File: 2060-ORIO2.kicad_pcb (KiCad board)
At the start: 4 copper layers, 99 x 99 mm, 159 parts, among them J1 TBL001-500-02GY-2GY, J101 RaspberryPI-B+header, J133 Conn_02x05_Odd_Even, J134 Conn_01x04, J301 Conn_01x08, J302 Conn_01x08, J303 Conn_01x08, J304 Conn_01x08, J305 Conn_01x08, J306 Conn_01x08, J307 Conn_01x08, J308 Conn_01x08, J321 Conn_01x08, J322 Conn_01x08, J323 Conn_01x08, J331 Conn_01x08, J332 Conn_01x08, J333 Conn_01x08, J341 Conn_01x10, J342 Conn_01x10, J343 Conn_01x10, J35 Conn_01x02, J351 Conn_01x10, J352 Conn_01x10, J353 Conn_01x10, J354 Conn_01x10, Q101 DMG2305UX-13, Q102 ULN2803ADWR, Q103 DMMT5401, SW101 SW_DIP_x08, U1 TPS563231, U10 SN74LVC4245AN, U102 AZ1117CH-3.3TRG1, U103 AZ1117CH-1.2, U104 ICE40HX4K-TQ144, U105 MCP3008, U11 AZ1117CH-3.3TRG1, U12 AP3012, U2 TPS563231, U3 SN74LVC4245AN, U4 SN74LVC4245AN, U5 SN74LVC4245AN, U6 SN74LVC4245AN, U7 SN74LVC4245AN, U8 TPS563231, U9 SN74LVC4245AN, Y101 XLH536025_000000I

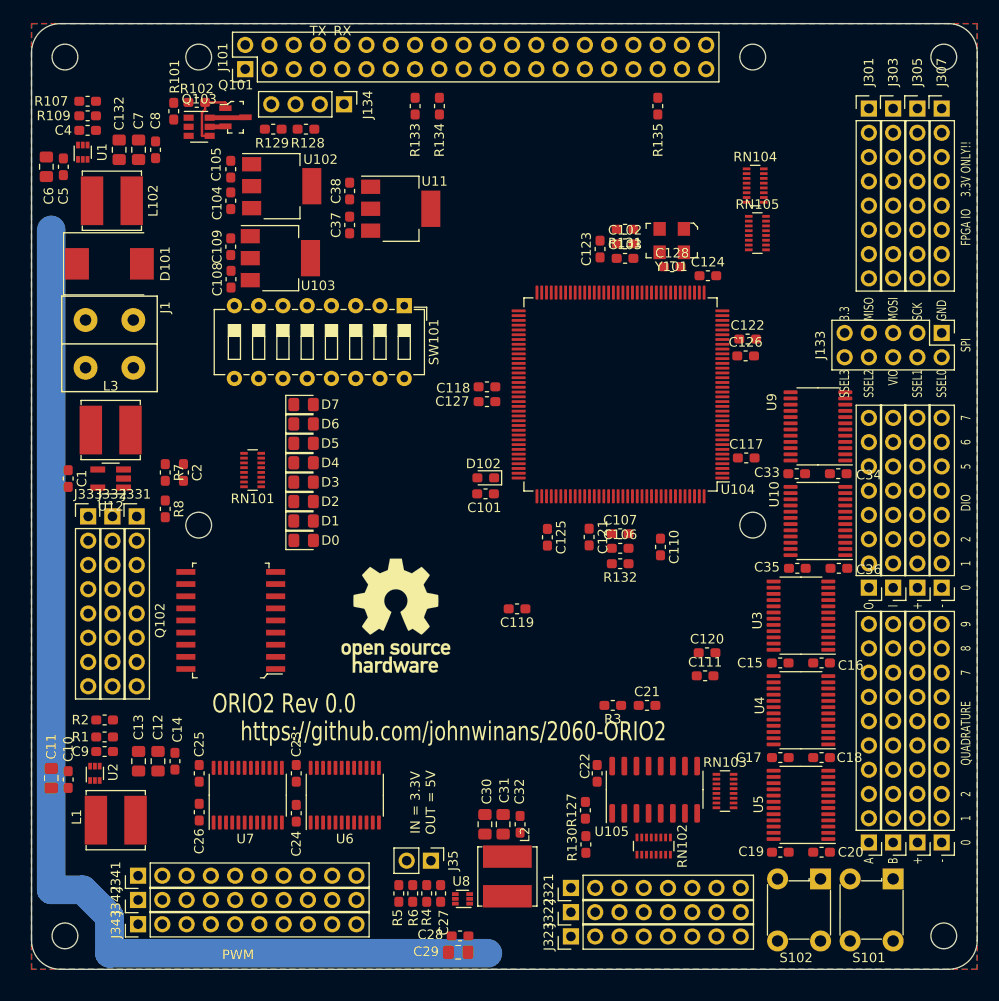
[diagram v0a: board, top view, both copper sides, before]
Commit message: checkpoint
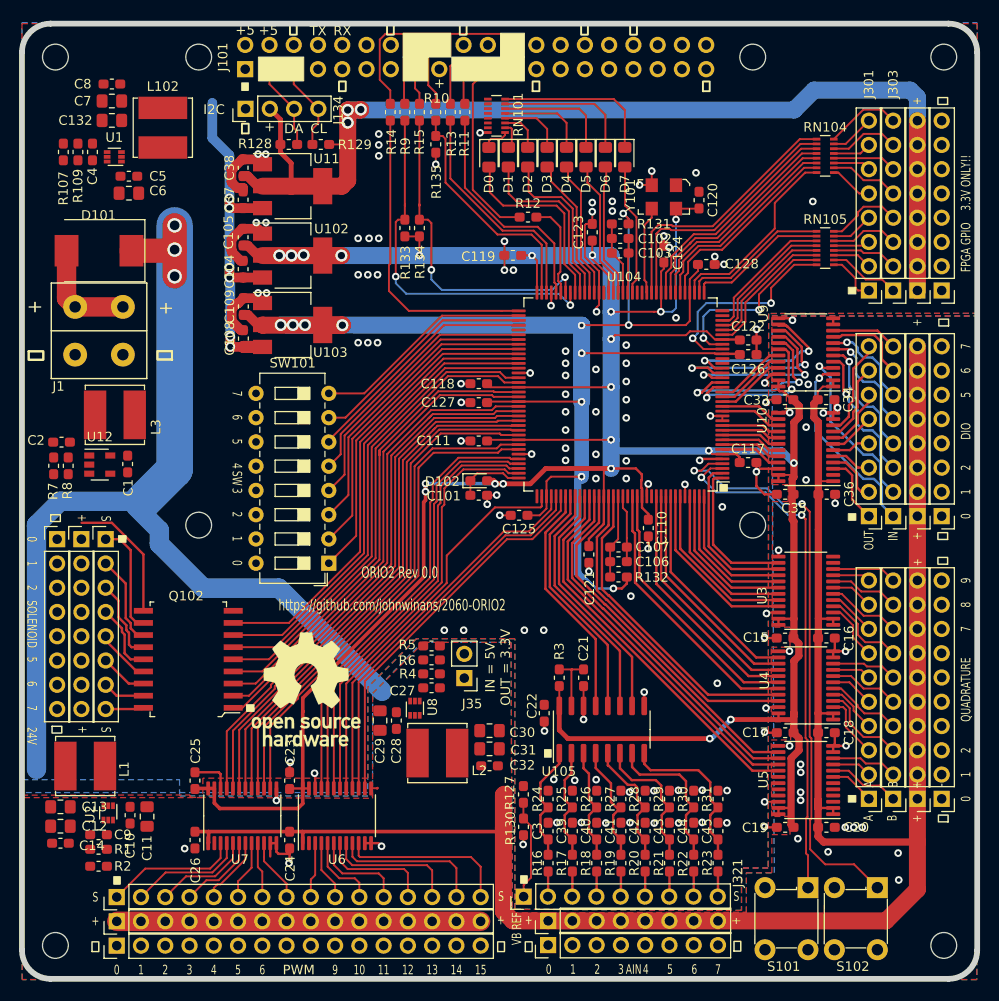
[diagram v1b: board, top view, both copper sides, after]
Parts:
- removed J133: Conn_02x05_Odd_Even, Connector_PinHeader_2.54mm:PinHeader_2x05_P2.54mm_Vertical
- removed Q101: DMG2305UX-13, digikey-footprints:SOT-23-3
- removed Q103: DMMT5401, Package_TO_SOT_SMD:SOT-23-6
- removed R101, R102: 22, Resistor_SMD:R_0603_1608Metric_Pad1.05x0.95mm_HandSolder
- removed RN102, RN103: R_Pack08, Resistor_SMD:R_Array_Convex_8x0602
- added C3: X, Capacitor_SMD:C_0603_1608Metric_Pad1.05x0.95mm_HandSolder, F.Cu at (127.1, 126.5)
- added C39: X, Capacitor_SMD:C_0603_1608Metric_Pad1.05x0.95mm_HandSolder, F.Cu at (129.6, 126.5)
- added C40: X, Capacitor_SMD:C_0603_1608Metric_Pad1.05x0.95mm_HandSolder, F.Cu at (132.2, 126.5)
- added C41: X, Capacitor_SMD:C_0603_1608Metric_Pad1.05x0.95mm_HandSolder, F.Cu at (134.7, 126.5)
- added C42: X, Capacitor_SMD:C_0603_1608Metric_Pad1.05x0.95mm_HandSolder, F.Cu at (137.2, 126.5)
- added C43: X, Capacitor_SMD:C_0603_1608Metric_Pad1.05x0.95mm_HandSolder, F.Cu at (139.8, 126.5)
- added C44: X, Capacitor_SMD:C_0603_1608Metric_Pad1.05x0.95mm_HandSolder, F.Cu at (142.3, 126.5)
- added C45: X, Capacitor_SMD:C_0603_1608Metric_Pad1.05x0.95mm_HandSolder, F.Cu at (144.9, 126.5)
- added R10: X, Resistor_SMD:R_0603_1608Metric_Pad1.05x0.95mm_HandSolder, F.Cu at (115.3, 51.3)
- added R11: X, Resistor_SMD:R_0603_1608Metric_Pad1.05x0.95mm_HandSolder, F.Cu at (118.4, 51.3)
- added R12: X, Resistor_SMD:R_0603_1608Metric_Pad1.05x0.95mm_HandSolder, F.Cu at (125.0, 62.3)
- added R13: X, Resistor_SMD:R_0603_1608Metric_Pad1.05x0.95mm_HandSolder, F.Cu at (116.8, 51.3)
- added R14: X, Resistor_SMD:R_0603_1608Metric_Pad1.05x0.95mm_HandSolder, F.Cu at (110.6, 51.3)
- added R15: X, Resistor_SMD:R_0603_1608Metric_Pad1.05x0.95mm_HandSolder, F.Cu at (113.6, 51.3)
- added R16: X, Resistor_SMD:R_0603_1608Metric_Pad1.05x0.95mm_HandSolder, F.Cu at (127.1, 129.9)
- added R17: X, Resistor_SMD:R_0603_1608Metric_Pad1.05x0.95mm_HandSolder, F.Cu at (129.6, 129.9)
- added R18: X, Resistor_SMD:R_0603_1608Metric_Pad1.05x0.95mm_HandSolder, F.Cu at (132.2, 129.9)
- added R19: X, Resistor_SMD:R_0603_1608Metric_Pad1.05x0.95mm_HandSolder, F.Cu at (134.7, 129.9)
- added R20: X, Resistor_SMD:R_0603_1608Metric_Pad1.05x0.95mm_HandSolder, F.Cu at (137.2, 129.9)
- added R21: X, Resistor_SMD:R_0603_1608Metric_Pad1.05x0.95mm_HandSolder, F.Cu at (139.8, 129.9)
- added R22: X, Resistor_SMD:R_0603_1608Metric_Pad1.05x0.95mm_HandSolder, F.Cu at (142.3, 129.9)
- added R23: X, Resistor_SMD:R_0603_1608Metric_Pad1.05x0.95mm_HandSolder, F.Cu at (144.9, 129.9)
- added R24: X, Resistor_SMD:R_0603_1608Metric_Pad1.05x0.95mm_HandSolder, F.Cu at (127.1, 123.2)
- added R25: X, Resistor_SMD:R_0603_1608Metric_Pad1.05x0.95mm_HandSolder, F.Cu at (129.6, 123.2)
- added R26: X, Resistor_SMD:R_0603_1608Metric_Pad1.05x0.95mm_HandSolder, F.Cu at (132.2, 123.2)
- added R27: X, Resistor_SMD:R_0603_1608Metric_Pad1.05x0.95mm_HandSolder, F.Cu at (134.7, 123.2)
- added R28: X, Resistor_SMD:R_0603_1608Metric_Pad1.05x0.95mm_HandSolder, F.Cu at (137.2, 123.2)
- added R29: X, Resistor_SMD:R_0603_1608Metric_Pad1.05x0.95mm_HandSolder, F.Cu at (139.8, 123.2)
- added R30: X, Resistor_SMD:R_0603_1608Metric_Pad1.05x0.95mm_HandSolder, F.Cu at (142.3, 123.2)
- added R31: X, Resistor_SMD:R_0603_1608Metric_Pad1.05x0.95mm_HandSolder, F.Cu at (144.9, 123.2)
- added R9: X, Resistor_SMD:R_0603_1608Metric_Pad1.05x0.95mm_HandSolder, F.Cu at (112.1, 51.3)
- J321: value Conn_01x08 -> Conn_01x09; footprint Connector_PinHeader_2.54mm:PinHeader_1x08_P2.54mm_Vertical -> Connector_PinHeader_2.54mm:PinHeader_1x09_P2.54mm_Vertical
- J341, J342, J343: value Conn_01x10 -> Conn_01x16; footprint Connector_PinHeader_2.54mm:PinHeader_1x10_P2.54mm_Vertical -> Connector_PinHeader_2.54mm:PinHeader_1x16_P2.54mm_Vertical
- U12: footprint Package_TO_SOT_SMD:SOT-23-5_HandSoldering -> Package_TO_SOT_SMD:SOT-23-5
- moved C120 47.4 mm to (142.9, 60.5), turned to 90 degrees
- moved RN101 45.0 mm to (121.7, 51.7)
- moved D0 44.6 mm to (120.9, 56.0), turned to 270 degrees
- moved D1 43.7 mm to (122.9, 56.0), turned to 270 degrees
- moved D2 43.0 mm to (124.9, 56.0), turned to 270 degrees
- moved D3 42.5 mm to (127.0, 56.0), turned to 270 degrees
- moved D7 42.4 mm to (135.1, 56.0), turned to 270 degrees
- moved D4 42.2 mm to (129.0, 56.0), turned to 270 degrees
- moved D6 42.2 mm to (133.1, 56.0), turned to 270 degrees
- moved D5 42.1 mm to (131.0, 56.0), turned to 270 degrees
- moved C119 37.0 mm to (123.4, 66.3)
- moved C111 34.1 mm to (119.8, 85.7), turned to 180 degrees
- moved SW101 28.1 mm to (104.1, 98.5), turned to 180 degrees
- moved R5 26.1 mm to (114.9, 107.2), turned to 0 degrees
- moved C29 25.6 mm to (109.5, 115.0), turned to 270 degrees
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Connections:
- net /IOT_197 renamed Net-(U104-Pad128)
- net Net-(J301-Pad6) renamed /FIO10
- net Net-(J303-Pad3) renamed /FIO5
- C22 pad 1: VCC_IO -> +3V3
- J101 pad 16: /CDONE -> /GPIO23
- J101 pad 18: /~CRESET~ -> /GPIO24
- J101 pad 19: /FPGA_MOSI -> /SPI_MOSI
- J101 pad 21: /FPGA_MISO -> /SPI_MISO
- J101 pad 23: /FPGA_SCLK -> /SPI_SCLK
- J101 pad 36: /FPGA_SSEL -> /GPIO16
- J301 pad 1: Net-(J301-Pad1) -> /FIO0
- J301 pad 2: Net-(J301-Pad2) -> /FIO2
- J301 pad 3: Net-(J301-Pad3) -> /FIO4
- J301 pad 4: Net-(J301-Pad4) -> /FIO6
- J301 pad 5: Net-(J301-Pad5) -> /FIO8
- J301 pad 7: Net-(J301-Pad7) -> /FIO12
- J301 pad 8: Net-(J301-Pad8) -> /FIO14
- J303 pad 1: Net-(J303-Pad1) -> /FIO1
- J303 pad 2: Net-(J303-Pad2) -> /FIO3
- J303 pad 4: Net-(J303-Pad4) -> /FIO7
- J303 pad 5: Net-(J303-Pad5) -> /FIO9
- J303 pad 6: Net-(J303-Pad6) -> /FIO11
- J303 pad 7: Net-(J303-Pad7) -> /FIO13
- J303 pad 8: Net-(J303-Pad8) -> /FIO15
- J321 pad 1: Net-(J321-Pad1) -> /VBATT_DIV
- J35 pad 1: VCC_IO -> Net-(J35-Pad1)
- J35 pad 2: Net-(J35-Pad2) -> GND
- J351 pad 4: /Qa3 -> /QA3
- R127 pad 1: /ADC0_11 -> /VBATT_DIV
- R130 pad 2: /ADC0_11 -> /VBATT_DIV
- R135 pad 2: /FPGA_SSEL -> /FPGA_SS
- R3 pad 2: VCC_IO -> +3V3
- R6 pad 1: Net-(J35-Pad2) -> Net-(J35-Pad1)
- RN104 pad 1: Net-(RN104-Pad1) -> /IOB_80
- RN104 pad 10: Net-(J301-Pad7) -> /FIO9
- RN104 pad 12: Net-(J301-Pad5) -> /FIO11
- RN104 pad 13: Net-(J301-Pad4) -> /FIO12
- RN104 pad 14: Net-(J301-Pad3) -> /FIO13
- RN104 pad 15: Net-(J301-Pad2) -> /FIO14
- RN104 pad 16: Net-(J301-Pad1) -> /FIO15
- RN104 pad 2: Net-(RN104-Pad2) -> /IOB_79
- RN104 pad 3: Net-(RN104-Pad3) -> /IOB_73
- RN104 pad 4: Net-(RN104-Pad4) -> /IOB_72
- RN104 pad 5: Net-(RN104-Pad5) -> /IOB_71
- RN104 pad 6: Net-(RN104-Pad6) -> /IOB_64
- RN104 pad 7: Net-(RN104-Pad7) -> /IOB_63
- RN104 pad 8: Net-(RN104-Pad8) -> /IOB_61
- RN104 pad 9: Net-(J301-Pad8) -> /FIO8
- RN105 pad 1: Net-(RN105-Pad1) -> /IOB_57
- RN105 pad 10: Net-(J303-Pad7) -> /FIO1
- RN105 pad 11: Net-(J303-Pad6) -> /FIO2
- RN105 pad 12: Net-(J303-Pad5) -> /FIO3
- RN105 pad 13: Net-(J303-Pad4) -> /FIO4
- RN105 pad 15: Net-(J303-Pad2) -> /FIO6
- RN105 pad 16: Net-(J303-Pad1) -> /FIO7
- RN105 pad 2: Net-(RN105-Pad2) -> /IOB_56
- RN105 pad 3: Net-(RN105-Pad3) -> /IOL_25B
- RN105 pad 4: Net-(RN105-Pad4) -> /IOL_25A
- RN105 pad 5: Net-(RN105-Pad5) -> /IOL_24B
- RN105 pad 6: Net-(RN105-Pad6) -> /IOL_24A
- RN105 pad 7: Net-(RN105-Pad7) -> /IOL_23B
- RN105 pad 8: Net-(RN105-Pad8) -> /IOL_23A
- RN105 pad 9: Net-(J303-Pad8) -> /FIO0
- S101 pad 1: /IOT_220 -> /PB0
- S101 pad 4: GND -> Net-(S101-Pad4)
- S102 pad 1: /IOT_219 -> /PB1
- S102 pad 4: GND -> Net-(S102-Pad4)
- SW101 pad 1: /SW7 -> /SW0
- SW101 pad 2: /SW6 -> /SW1
- SW101 pad 3: /SW5 -> /SW2
- SW101 pad 4: /SW4 -> /SW3
- SW101 pad 5: /SW3 -> /SW4
- SW101 pad 6: /SW2 -> /SW5
- SW101 pad 7: /SW1 -> /SW6
- SW101 pad 8: /SW0 -> /SW7
- U10 pad 14: Net-(U10-Pad14) -> /FPGA_DOUT7
- U10 pad 15: Net-(U10-Pad15) -> /FPGA_DOUT6
- U10 pad 16: Net-(U10-Pad16) -> /FPGA_DOUT5
- U10 pad 17: Net-(U10-Pad17) -> /FPGA_DOUT4
- U10 pad 18: Net-(U10-Pad18) -> /FPGA_DOUT3
- U10 pad 19: Net-(U10-Pad19) -> /FPGA_DOUT2
- U10 pad 20: Net-(U10-Pad20) -> /FPGA_DOUT1
- U10 pad 21: Net-(U10-Pad21) -> /FPGA_DOUT0
- U104 pad 1: /IOL_2A -> /FPGA_QB9
- U104 pad 10: /IOL_5B -> /FPGA_DOUT3
- U104 pad 101: /IOR_160 -> /FPGA_PWM6
- U104 pad 102: /IOR_161 -> /FPGA_PWM7
- U104 pad 104: /IOR_164 -> /FPGA_PWM8
- U104 pad 105: /IOR_165 -> /FPGA_PWM9
- U104 pad 106: /IOR_166 -> /FPGA_PWM10
- U104 pad 107: /IOR_167 -> /FPGA_PWM11
- U104 pad 11: /IOL_8A -> /FPGA_DOUT4
- U104 pad 110: /IOT_168 -> /FPGA_PWM12
- U104 pad 112: /IOT_169 -> /FPGA_PWM13
- U104 pad 113: /IOT_170 -> /FPGA_PWM14
- U104 pad 114: /IOT_171 -> /FPGA_PWM15
- U104 pad 115: /IOT_172 -> /ADC_CLK
- U104 pad 116: /IOT_173 -> /ADC_SO
- U104 pad 117: /IOT_174 -> /ADC_SI
- U104 pad 118: /IOT_177 -> /~ADC_CS
- U104 pad 119: /IOT_178 -> /FPGA_QA0
- U104 pad 12: /IOL_8B -> /FPGA_DOUT5
- U104 pad 120: /IOT_179 -> /FPGA_QB0
- U104 pad 121: /IOT_181 -> /FPGA_QA1
- U104 pad 122: /IOT_190 -> /FPGA_QB1
- U104 pad 124: /IOT_191 -> /FPGA_QA2
- U104 pad 125: /IOT_192 -> /FPGA_QB2
- U104 pad 129: /IOT_198 -> /FPGA_QA3
- U104 pad 130: /IOT_206 -> /FPGA_QB3
- U104 pad 134: /IOT_212 -> /FPGA_QA4
- U104 pad 135: /IOT_213 -> /FPGA_QB4
- U104 pad 136: /IOT_214 -> /FPGA_QA5
- U104 pad 137: /IOT_215 -> /FPGA_QB5
- U104 pad 138: /IOT_216 -> /FPGA_QA6
- U104 pad 139: /IOT_217 -> /FPGA_QB6
- U104 pad 141: /IOT_219 -> /FPGA_QA7
- U104 pad 142: /IOT_220 -> /FPGA_QB7
- U104 pad 143: /IOT_221 -> /FPGA_QA8
- U104 pad 144: /IOT_222 -> /FPGA_QB8
- U104 pad 15: /IOL_10A -> /FPGA_DOUT6
- U104 pad 16: /IOL_10B -> /FPGA_DOUT7
- U104 pad 17: /IOL_12A -> /FPGA_DIN0
- U104 pad 18: /IOL_12B -> /FPGA_DIN1
- U104 pad 19: /IOL_13A -> /FPGA_DIN2
- U104 pad 2: /IOL_2B -> /FPGA_QA9
- U104 pad 20: /IOL_13B -> /FPGA_DIN3
- U104 pad 21: /IOL_14A -> /FPGA_DIN4
- U104 pad 22: /IOL_14B -> /FPGA_DIN5
- U104 pad 23: /IOL_17A -> /FPGA_DIN6
- U104 pad 24: /IOL_17B -> /FPGA_DIN7
- U104 pad 3: /IOL_3A -> /PB0
- U104 pad 4: /IOL_3B -> /PB1
- U104 pad 52: /IOB_82 -> /LED_7
- U104 pad 55: /SPI_CE0 -> /LED_6
- U104 pad 56: /IOB_94 -> /LED_5
- U104 pad 60: /IOB_95 -> /LED_4
- U104 pad 61: /IOB_96 -> /LED_3
- U104 pad 62: /IOB_102 -> /LED_2
- U104 pad 63: /IOB_103 -> /LED_1
- U104 pad 64: /IOB_104 -> /LED_0
- U104 pad 67: /FPGA_MISO -> /FPGA_SDO
- U104 pad 68: /FPGA_MOSI -> /FPGA_SDI
- U104 pad 7: /IOL_4A -> /FPGA_DOUT0
- U104 pad 70: /FPGA_SCLK -> /FPGA_SCK
- U104 pad 71: /FPGA_SSEL -> /FPGA_SS
- U104 pad 73: /IOR_109 -> /FPGA_CE0
- U104 pad 74: /IOR_110 -> /SW7
- U104 pad 75: /IOR_111 -> /SW6
- U104 pad 76: /IOR_112 -> /SW5
- U104 pad 78: /IOR_114 -> /SW4
- U104 pad 79: /IOR_115 -> /SW3
- U104 pad 8: /IOL_4B -> /FPGA_DOUT1
- U104 pad 80: /IOR_116 -> /SW2
- U104 pad 81: /IOR_117 -> /SW1
- U104 pad 82: /IOR_118 -> /SW0
- U104 pad 83: /IOR_119 -> /SOL_7
- U104 pad 84: /IOR_120 -> /SOL_6
- U104 pad 85: /IOR_128 -> /SOL_5
- U104 pad 87: /IOR_136 -> /SOL_4
- U104 pad 88: /IOR_137 -> /SOL_3
- U104 pad 9: /IOL_5A -> /FPGA_DOUT2
- U104 pad 90: /IOR_138 -> /SOL_2
- U104 pad 91: /IOR_139 -> /SOL_1
- U104 pad 93: /IOR_140 -> /SOL_0
- U104 pad 94: /IOR_141 -> /FPGA_PWM0
- U104 pad 95: /IOR_144 -> /FPGA_PWM1
- U104 pad 96: /IOR_146 -> /FPGA_PWM2
- U104 pad 97: /IOR_147 -> /FPGA_PWM3
- U104 pad 98: /IOR_148 -> /FPGA_PWM4
- U104 pad 99: /IOR_152 -> /FPGA_PWM5
- U105 pad 10: Net-(U105-Pad10) -> /~ADC_CS
- U105 pad 11: Net-(U105-Pad11) -> /ADC_SI
- U105 pad 12: Net-(U105-Pad12) -> /ADC_SO
- U105 pad 13: Net-(U105-Pad13) -> /ADC_CLK
- U105 pad 16: VCC_IO -> +3V3
- U3 pad 10: Net-(U3-Pad10) -> /QB9
- U3 pad 14: Net-(U3-Pad14) -> /FPGA_QB9
- U3 pad 15: Net-(U3-Pad15) -> /FPGA_QA9
- U3 pad 16: Net-(U3-Pad16) -> /FPGA_QB8
- U3 pad 17: Net-(U3-Pad17) -> /FPGA_QA8
- U3 pad 18: Net-(U3-Pad18) -> /FPGA_QB7
- U3 pad 19: Net-(U3-Pad19) -> /FPGA_QA7
- U3 pad 20: Net-(U3-Pad20) -> /FPGA_QB6
- U3 pad 21: Net-(U3-Pad21) -> /FPGA_QA6
- U3 pad 3: Net-(U3-Pad3) -> /QA6
- U3 pad 4: Net-(U3-Pad4) -> /QB6
- U3 pad 5: Net-(U3-Pad5) -> /QA7
- U3 pad 6: Net-(U3-Pad6) -> /QB7
- U3 pad 7: Net-(U3-Pad7) -> /QA8
- U3 pad 8: Net-(U3-Pad8) -> /QB8
- U3 pad 9: Net-(U3-Pad9) -> /QA9
- U4 pad 10: Net-(U4-Pad10) -> /QB5
- U4 pad 14: Net-(U4-Pad14) -> /FPGA_QB5
- U4 pad 15: Net-(U4-Pad15) -> /FPGA_QA5
- U4 pad 16: Net-(U4-Pad16) -> /FPGA_QB4
- U4 pad 17: Net-(U4-Pad17) -> /FPGA_QA4
- U4 pad 18: Net-(U4-Pad18) -> /FPGA_QB3
- U4 pad 19: Net-(U4-Pad19) -> /FPGA_QA3
- U4 pad 20: Net-(U4-Pad20) -> /FPGA_QB2
- U4 pad 21: Net-(U4-Pad21) -> /FPGA_QA2
- U4 pad 3: Net-(U4-Pad3) -> /QA2
- U4 pad 4: Net-(U4-Pad4) -> /QB2
- U4 pad 5: Net-(U4-Pad5) -> /QA3
- U4 pad 6: Net-(U4-Pad6) -> /QB3
- U4 pad 7: Net-(U4-Pad7) -> /QA4
- U4 pad 8: Net-(U4-Pad8) -> /QB4
- U4 pad 9: Net-(U4-Pad9) -> /QA5
- U5 pad 10: Net-(U5-Pad10) -> /QB1
- U5 pad 14: Net-(U5-Pad14) -> /FPGA_QB1
- U5 pad 15: Net-(U5-Pad15) -> /FPGA_QA1
- U5 pad 16: Net-(U5-Pad16) -> /FPGA_QB0
- U5 pad 17: Net-(U5-Pad17) -> /FPGA_QA0
- U5 pad 7: Net-(U5-Pad7) -> /QA0
- U5 pad 8: Net-(U5-Pad8) -> /QB0
- U5 pad 9: Net-(U5-Pad9) -> /QA1
- U6 pad 10: Net-(U6-Pad10) -> /PWM15
- U6 pad 14: Net-(U6-Pad14) -> /FPGA_PWM15
- U6 pad 15: Net-(U6-Pad15) -> /FPGA_PWM14
- U6 pad 16: Net-(U6-Pad16) -> /FPGA_PWM13
- U6 pad 17: Net-(U6-Pad17) -> /FPGA_PWM12
- U6 pad 18: Net-(U6-Pad18) -> /FPGA_PWM11
- U6 pad 19: Net-(U6-Pad19) -> /FPGA_PWM10
- U6 pad 5: Net-(U6-Pad5) -> /PWM10
- U6 pad 6: Net-(U6-Pad6) -> /PWM11
- U6 pad 7: Net-(U6-Pad7) -> /PWM12
- U6 pad 8: Net-(U6-Pad8) -> /PWM13
- U6 pad 9: Net-(U6-Pad9) -> /PWM14
- U9 pad 14: Net-(U9-Pad14) -> /FPGA_DIN7
- U9 pad 15: Net-(U9-Pad15) -> /FPGA_DIN6
- U9 pad 16: Net-(U9-Pad16) -> /FPGA_DIN5
- U9 pad 17: Net-(U9-Pad17) -> /FPGA_DIN4
- U9 pad 18: Net-(U9-Pad18) -> /FPGA_DIN3
- U9 pad 19: Net-(U9-Pad19) -> /FPGA_DIN2
- U9 pad 20: Net-(U9-Pad20) -> /FPGA_DIN1
- U9 pad 21: Net-(U9-Pad21) -> /FPGA_DIN0
- Y101 pad 3: /IOB_82 -> /IOB_81
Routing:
- net +3V3: track 0.00 -> 356.2 mm, vias 0 -> 22
- net VCC_IO: track 0.00 -> 267.4 mm
- net +1V2: track 0.00 -> 144.3 mm, vias 0 -> 11
- net VCC_IO_3.3: track 0.00 -> 131.6 mm, vias 0 -> 3
- net GND: track 0.00 -> 125.3 mm, vias 0 -> 138
- net (no net): track 119.8 -> 0.00 mm
- net +BATT: track 0.00 -> 118.2 mm, vias 0 -> 3
- net /PB1: track 0.00 -> 61.3 mm, vias 0 -> 2
- net /FPGA_PWM0: track 0.00 -> 57.6 mm
- net /FPGA_PWM1: track 0.00 -> 56.4 mm
- net /FPGA_PWM2: track 0.00 -> 55.6 mm
- net /FPGA_PWM3: track 0.00 -> 55.2 mm
- net /PB0: track 0.00 -> 54.1 mm, vias 0 -> 2
- net /FPGA_PWM4: track 0.00 -> 54.1 mm
- net /FPGA_PWM5: track 0.00 -> 53.3 mm
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- removed copper zone on In1.Cu, net GND
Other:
- board size 99 x 99 mm -> 100 x 100 mm
- copper layers 4 -> 2
- net class Default: clearance 0.1524 -> 0.2032; trace_width 0.1524 -> 0.2032
- rule trace_clearance: 0.1524 -> 0.2032
- board text added: "+5"
- board text added: "10"
- board text added: "11"
- board text added: "12"
- board text added: "13"
- board text added: "14"
- board text added: "15"
- board text added: "24V"
- board text added: "3"
- board text added: "4"
- board text added: "AIN"
- board text added: "CL"
- board text added: "DA"
- board text added: "FPGA GPIO 3.3V ONLY!!"
- board text added: "I2C"
- board text added: "IN"
- board text added: "IN = 5V OUT = 3.3V"
- board text added: "OUT"
- board text added: "S"
- board text added: "SOLENOID"
- board text added: "SW"
- board text added: "VB REF"
- board text added: "⏚"
- board text removed: "3.3"
- board text removed: "FPGA IO 3.3V ONLY!!"
- board text removed: "GND"
- board text removed: "I"
- board text removed: "IN = 3.3V OUT = 5V"
- board text removed: "MISO"
- board text removed: "MOSI"
- board text removed: "O"
- board text removed: "SCK"
- board text removed: "SPI"
- board text removed: "SSEL0"
- board text removed: "SSEL1"
- board text removed: "SSEL2"
- board text removed: "SSEL3"
- board text removed: "VIO"
